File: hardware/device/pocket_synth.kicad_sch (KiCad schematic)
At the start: 7 parts

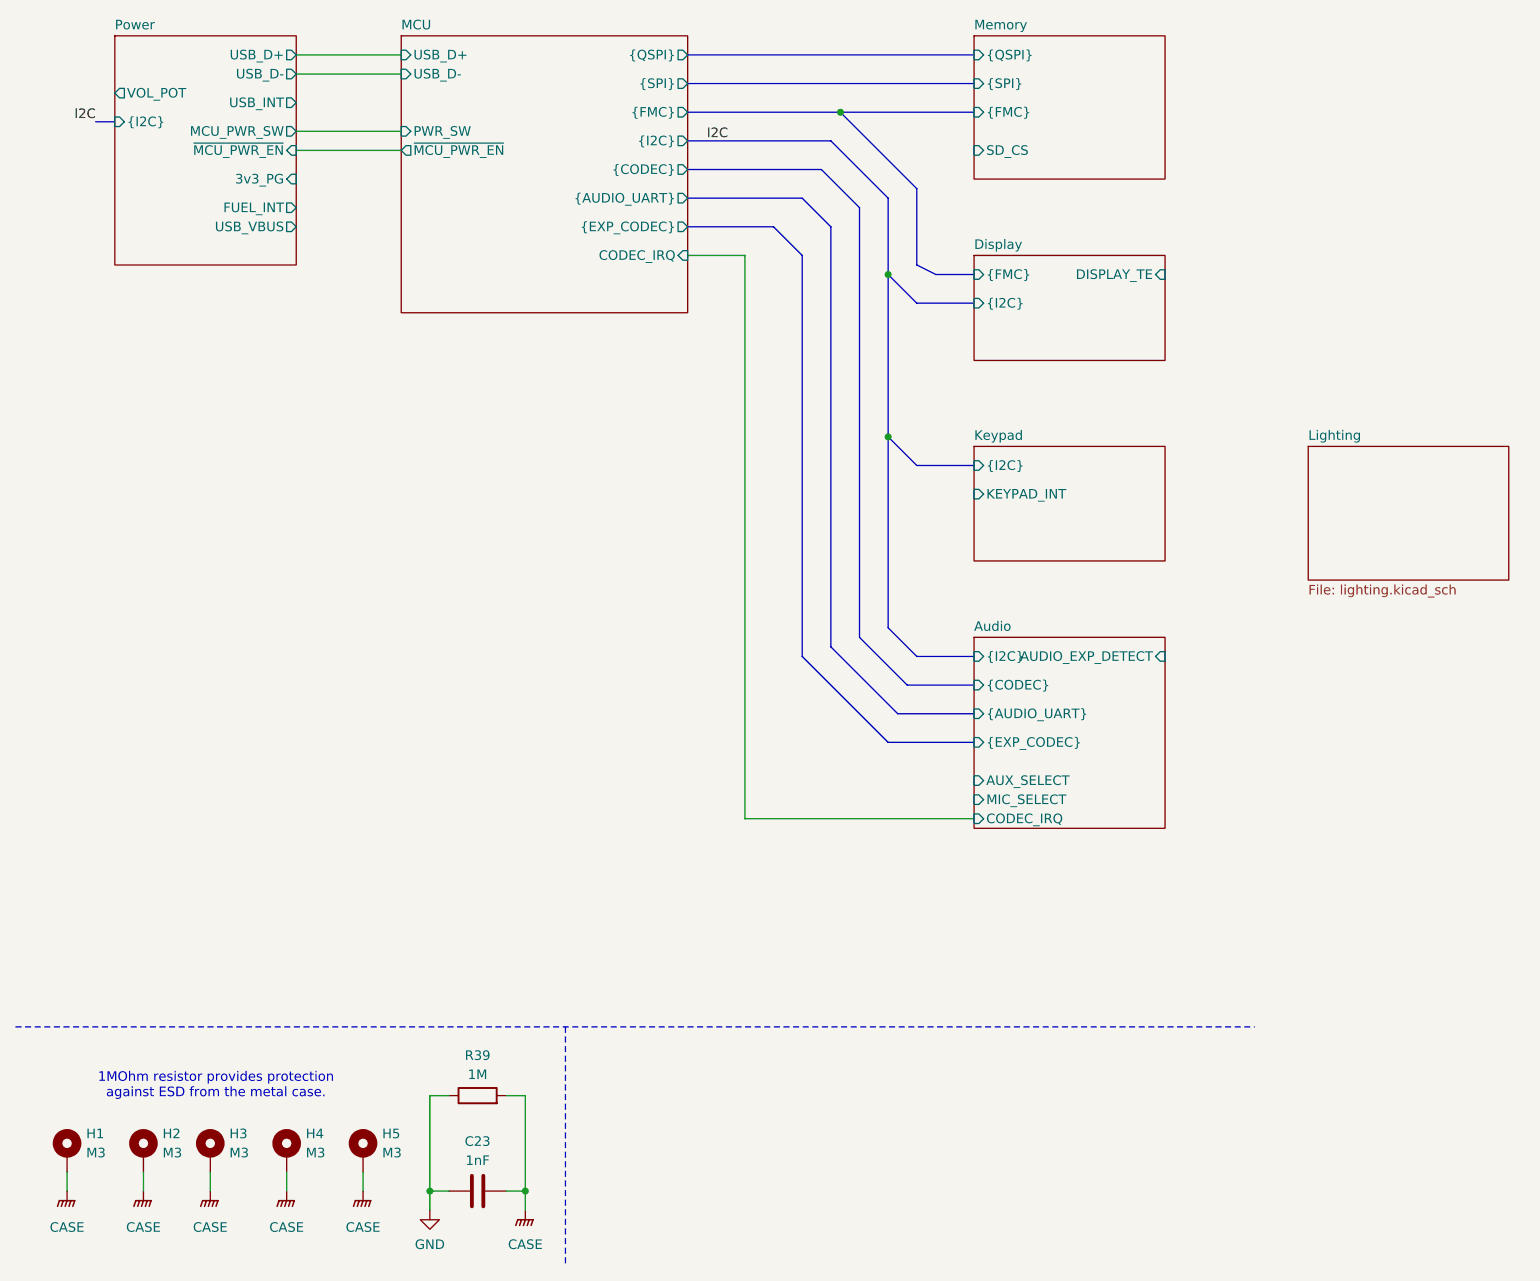
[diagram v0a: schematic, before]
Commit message: feat: audio system routing
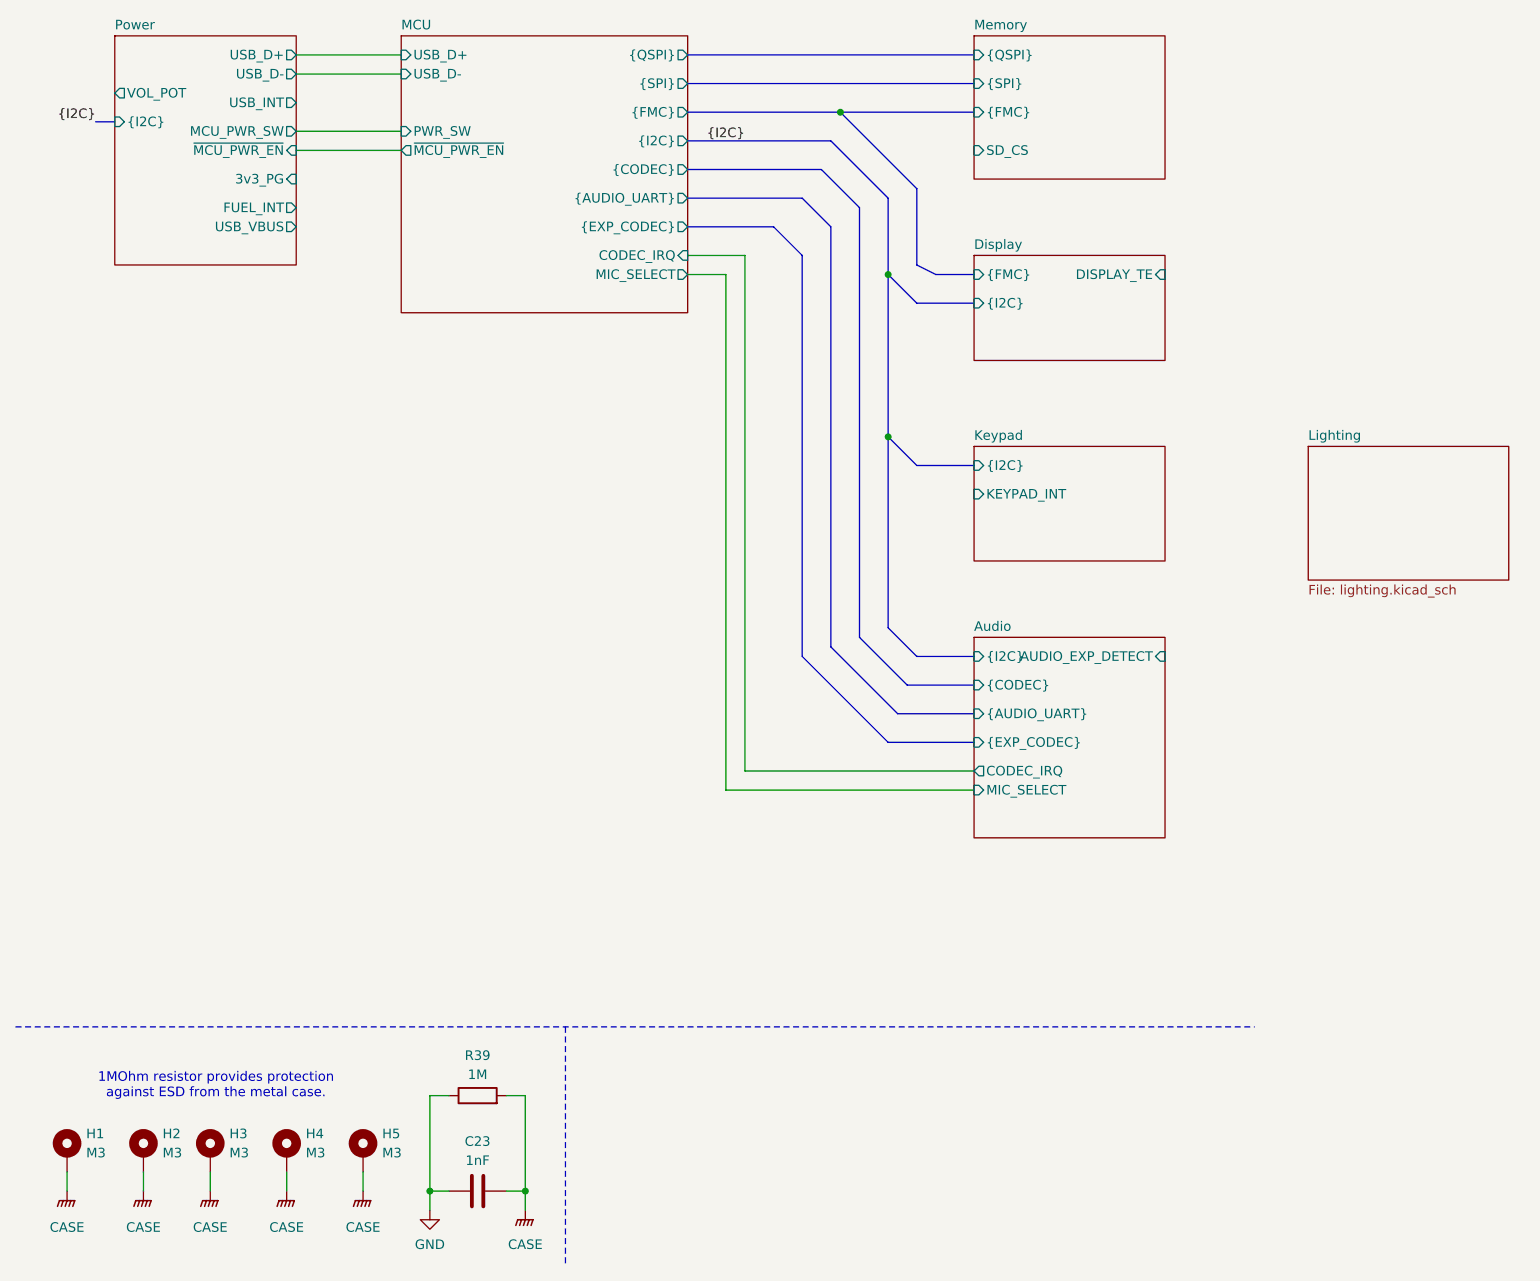
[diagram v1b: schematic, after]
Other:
- sheet Audio ports: added none; removed AUX_SELECT
- sheet MCU ports: added MIC_SELECT; removed none
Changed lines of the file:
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@@
+		)
+	)
+	(wire
+		(pts
+			(xy 106.68 134.62) (xy 139.7 134.62)
+		)
+		(stroke
+			(width 0)
+			(type default)
 		)
 	)
@@
 	(wire
 		(pts
-			(xy 109.22 63.5) (xy 109.22 138.43)
+			(xy 109.22 63.5) (xy 109.22 132.08)
 		)
 		(stroke
@@
 		)
 	)
+	(wire
+		(pts
+			(xy 101.6 66.04) (xy 106.68 66.04)
+		)
+		(stroke
+			(width 0)
+			(type default)
+		)
+	)
 	(bus
 		(pts
@@
 		(pts
 			(xy 101.6 59.69) (xy 113.03 59.69)
+		)
+		(stroke
+			(width 0)
+			(type default)
+		)
+	)
+	(wire
+		(pts
+			(xy 106.68 66.04) (xy 106.68 134.62)
 		)
 		(stroke
@@
 	(wire
 		(pts
-			(xy 109.22 138.43) (xy 139.7 138.43)
+			(xy 109.22 132.08) (xy 139.7 132.08)
 		)
 		(stroke
@@
 		)
 	)
-	(label "I2C"
+	(label "{I2C}"
 		(at 22.86 45.72 180)
 		(effects
@@
 		)
 	)
-	(label "I2C"
+	(label "{I2C}"
 		(at 104.14 48.26 0)
 		(effects
@@
 			)
 		)
+		(pin "MIC_SELECT" output
+			(at 101.6 66.04 0)
+			(effects
+				(font
+					(size 1.27 1.27)
+				)
+				(justify right)
+			)
+		)
 		(instances
 			(project "pocket_synth"
@@
 	(sheet
 		(at 139.7 114.3)
-		(size 25.4 25.4)
+		(size 25.4 26.67)
 		(exclude_from_sim no)
 		(in_bom yes)
@@
 		)
 		(property "Sheetfile" "audio.kicad_sch"
-			(at 139.7 140.2846 0)
+			(at 139.7 141.5546 0)
 			(effects
 				(font
@@
 			)
 		)
-		(pin "CODEC_IRQ" input
-			(at 139.7 138.43 180)
+		(pin "CODEC_IRQ" output
+			(at 139.7 132.08 180)
 			(effects
 				(font
@@
 			)
 		)
-		(pin "AUX_SELECT" input
-			(at 139.7 133.35 180)
-			(effects
-				(font
-					(size 1.27 1.27)
-				)
-				(justify left)
-			)
-		)
 		(pin "MIC_SELECT" input
-			(at 139.7 135.89 180)
-			(effects
-				(font
+			(at 139.7 134.62 180)
+			(effects
+				(font
